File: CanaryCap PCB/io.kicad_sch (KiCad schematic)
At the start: 15 parts, among them J1 USB_C_Receptacle_USB2.0_16P, J2 Conn_01x06_Pin, J3 Conn_01x04_Pin, U5 ADXL343

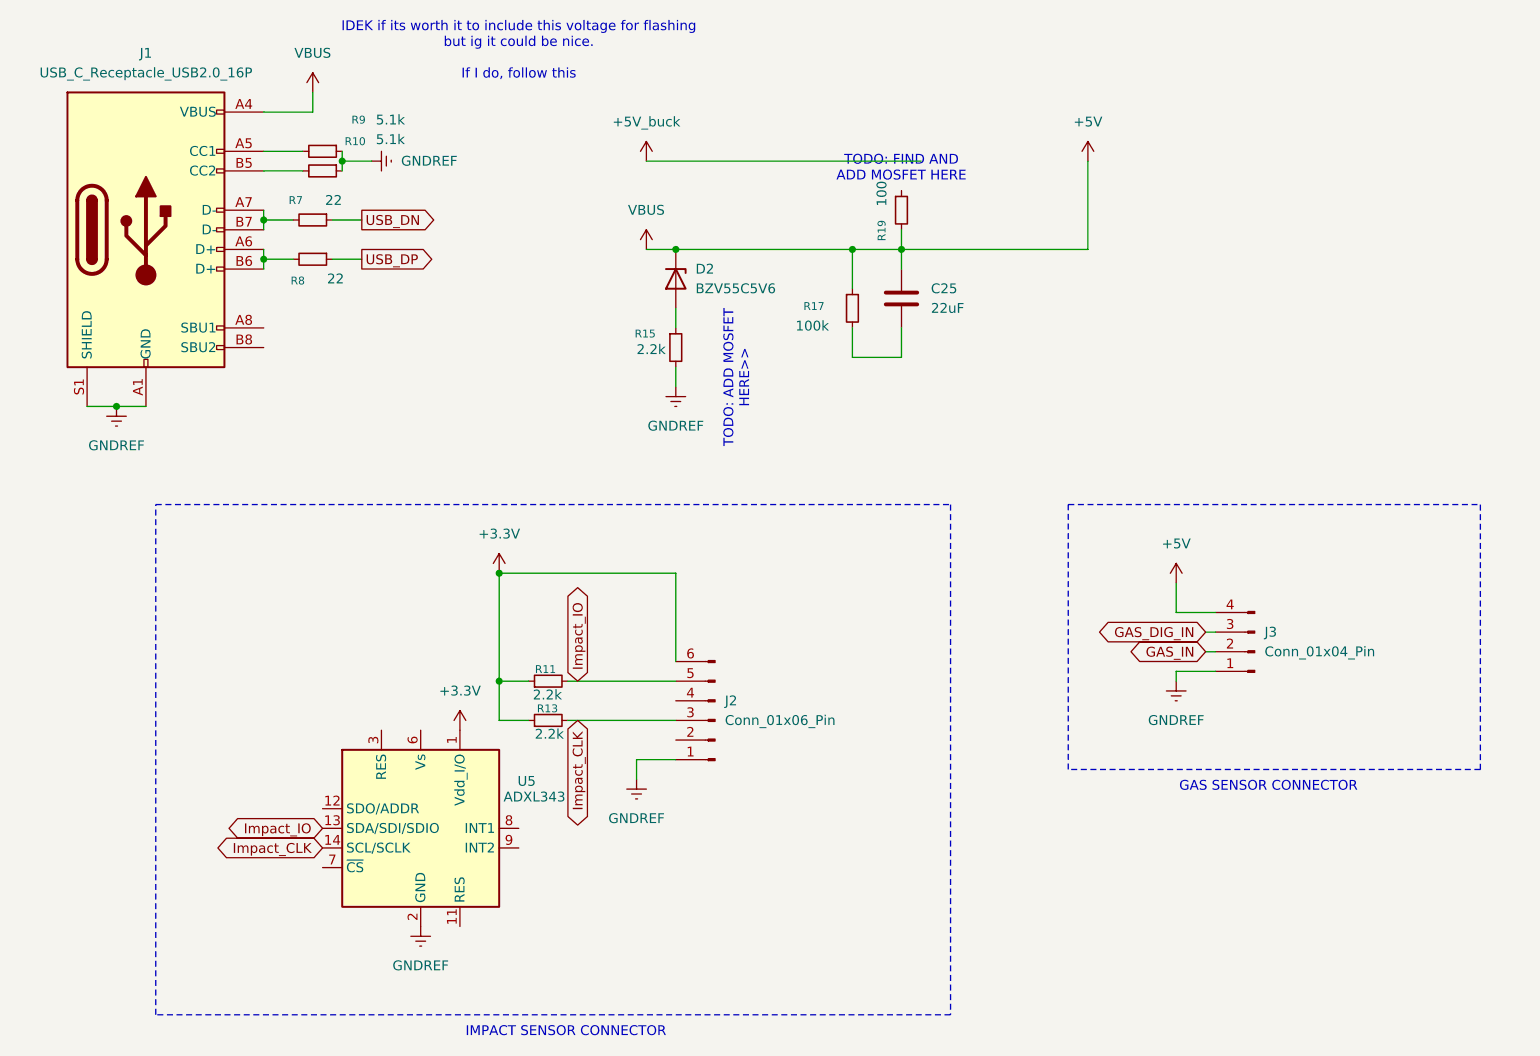
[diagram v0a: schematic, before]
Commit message: FIXED IT MF
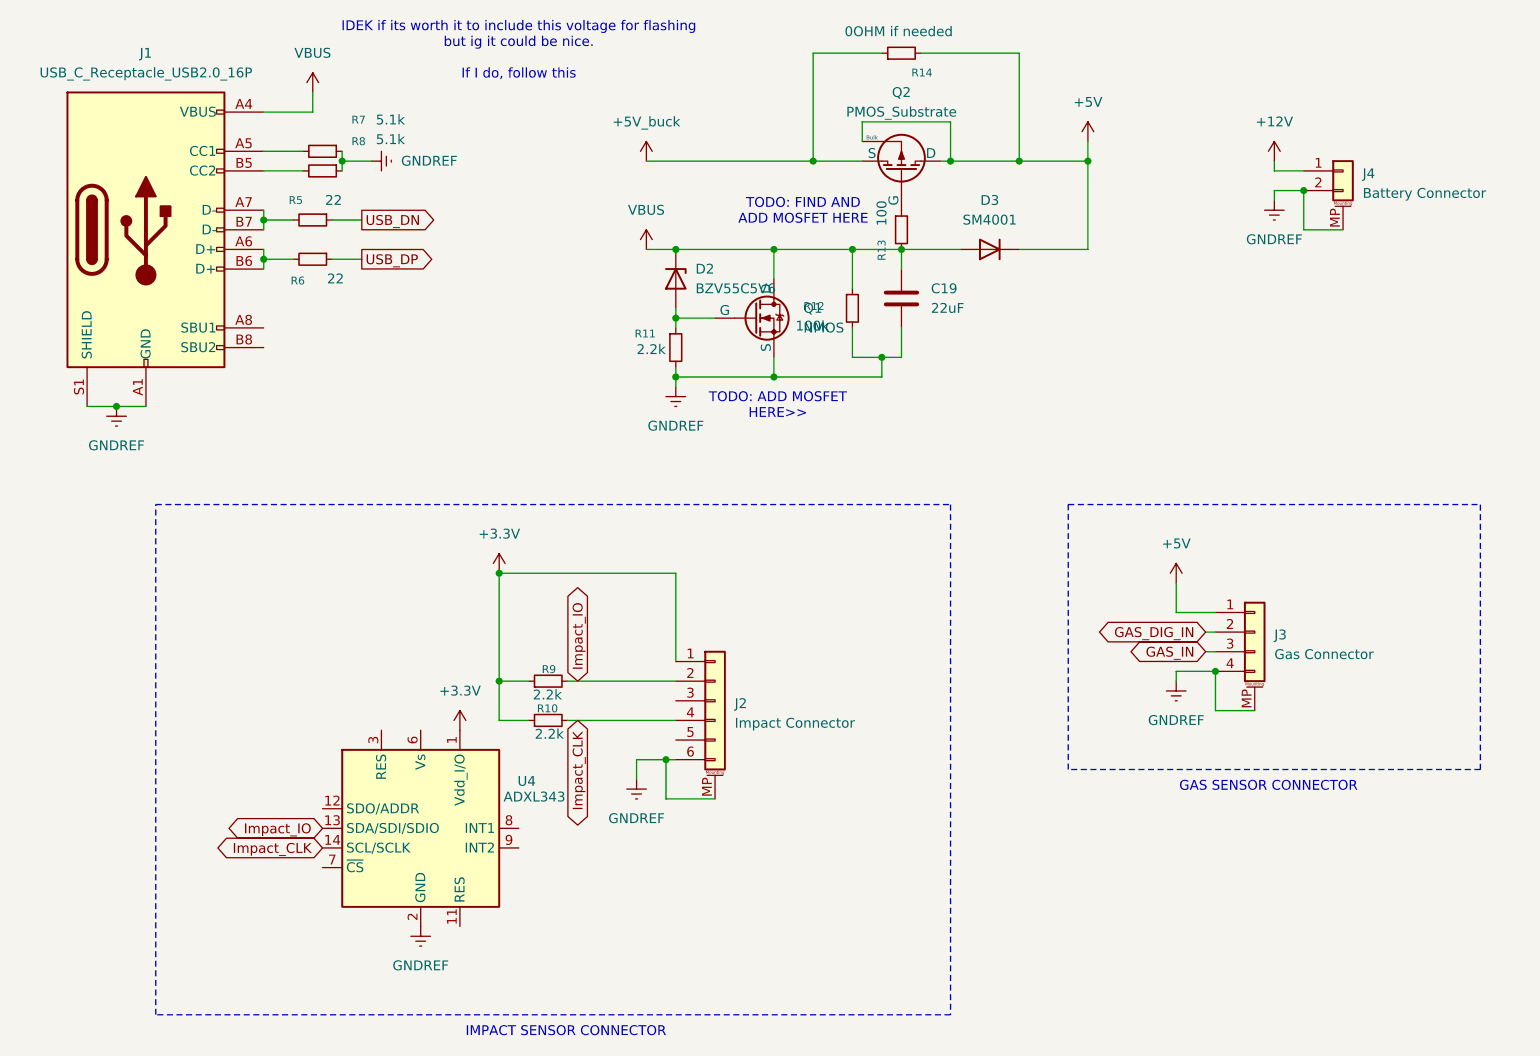
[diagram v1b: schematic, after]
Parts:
- removed J2: Conn_01x06_Pin, Connector_IDC:IDC-Header_2x03_P2.54mm_Vertical, symbol Connector:Conn_01x06_Pin
- removed J3: Conn_01x04_Pin, Connector_PinHeader_1.00mm:PinHeader_2x02_P1.00mm_Vertical, symbol Connector:Conn_01x04_Pin
- added D3: SM4001, Diode_SMD:D_MELF, symbol Diode:SM4001
- added J2: Impact Connector, Connector_Molex:Molex_CLIK-Mate_502443-0670_1x06-1MP_P2.00mm_Vertical, symbol Connector_Generic_MountingPin:Conn_01x06_MountingPin
- added J3: Gas Connector, Connector_Molex:Molex_CLIK-Mate_502443-0470_1x04-1MP_P2.00mm_Vertical, symbol Connector_Generic_MountingPin:Conn_01x04_MountingPin
- added J4: Battery Connector, Connector_Molex:Molex_CLIK-Mate_502443-0270_1x02-1MP_P2.00mm_Vertical, symbol Connector_Generic_MountingPin:Conn_01x02_MountingPin
- added Q1: NMOS, Package_TO_SOT_SMD:SOT-23, symbol Simulation_SPICE:NMOS
- added Q2: PMOS_Substrate, Package_TO_SOT_SMD:SOT-223, symbol Simulation_SPICE:PMOS_Substrate
- added R14: 0OHM if needed, Resistor_SMD:R_0603_1608Metric_Pad0.98x0.95mm_HandSolder, symbol Device:R_Small
- renumbered C25 to C19, R13 to R10, R15 to R11, R17 to R12, R19 to R13, R7 to R5, R8 to R6, R9 to R7, R10 to R8, R11 to R9, U5 to U4
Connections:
- net +3.3V: now also J2.1 (Pin_1)
- net +5V: now also D3.1 (K), J3.1 (Pin_1), Q2.2 (D), Q2.4 (Bulk), R14.2; no longer C19.1, D2.1 (K), J1.A4 (VBUS), J1.A9 (VBUS), J1.B4 (VBUS), J1.B9 (VBUS), R12.1, R13.2
- net +5V_buck: now also Q2.3 (S), R14.1
- net GAS_DIG_IN: now also J3.2 (Pin_2)
- net GAS_IN: now also J3.3 (Pin_3)
- net GNDREF: now also C19.2, R12.2, J2.6 (Pin_6), J2.MP (MountPin), J3.4 (Pin_4), J3.MP (MountPin), J4.2 (Pin_2), J4.MP (MountPin), Q1.2 (S)
- net Impact_CLK: now also J2.4 (Pin_4)
- net Impact_IO: now also J2.2 (Pin_2)
- net at D2.2 (A), R11.1: now also Q1.1 (G)
- net at R13.1: now also Q2.1 (G)
- new net +12V: J4.1 (Pin_1)
- new net VBUS: C19.1, D2.1 (K), D3.2 (A), J1.A4 (VBUS), J1.A9 (VBUS), J1.B4 (VBUS), J1.B9 (VBUS), Q1.3 (D), R12.1, R13.2
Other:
- moved on the sheet: R13

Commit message: Added todo
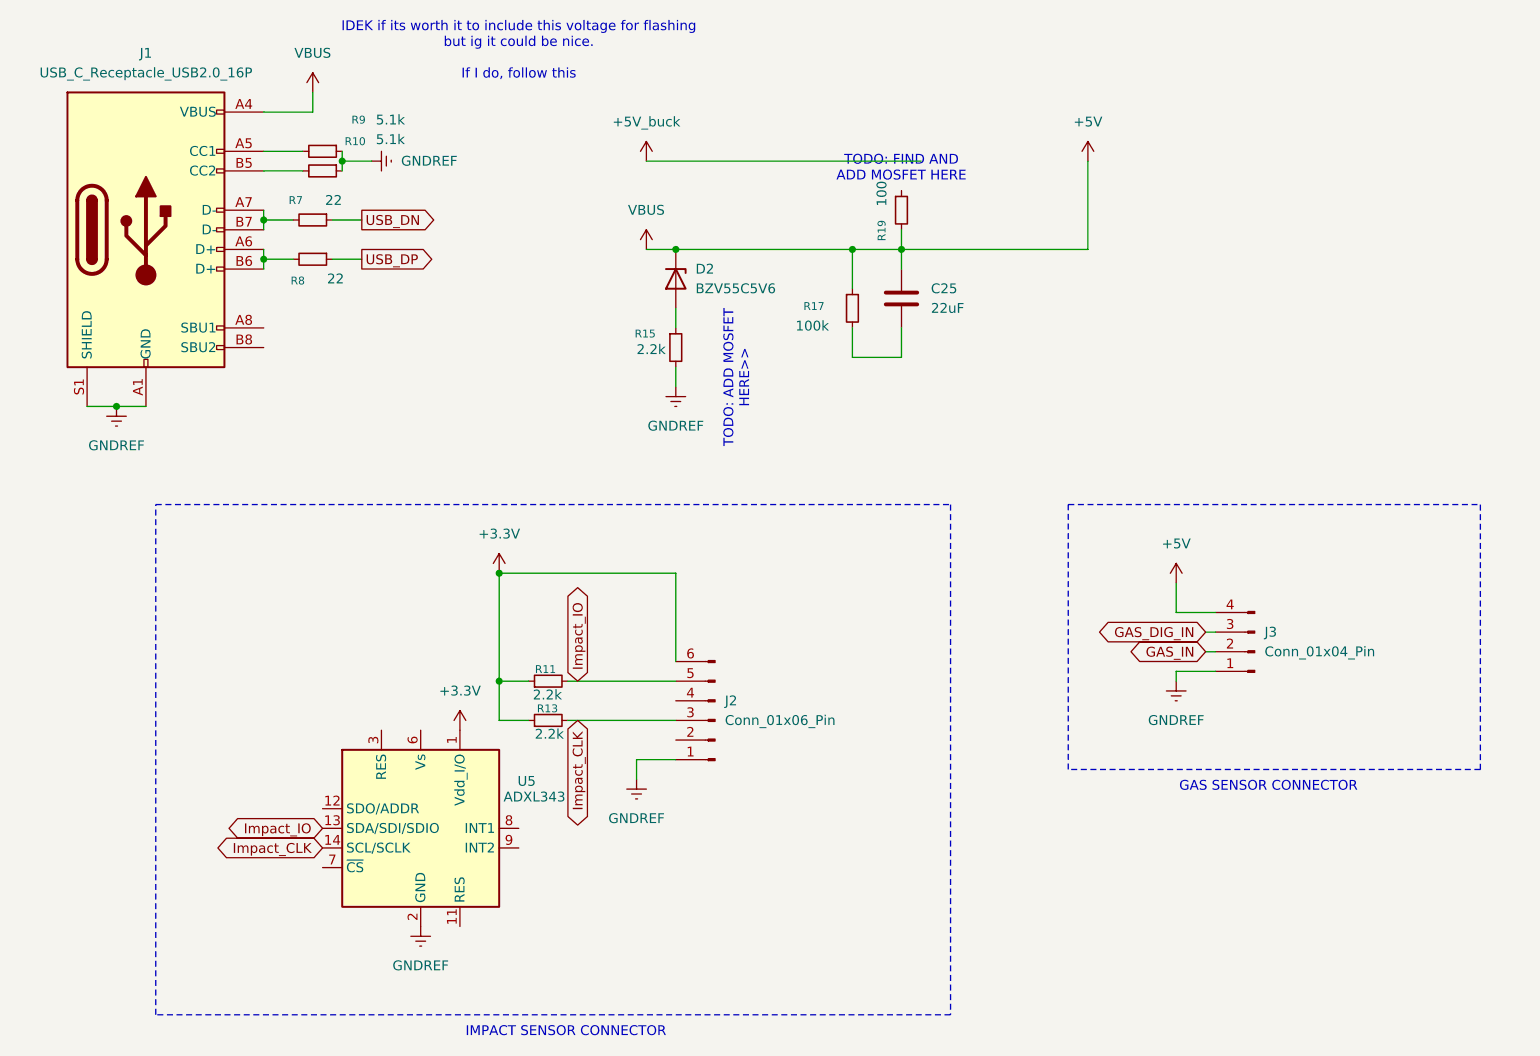
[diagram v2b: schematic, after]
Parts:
- removed D3: SM4001, Diode_SMD:D_MELF, symbol Diode:SM4001
- removed J2: Impact Connector, Connector_Molex:Molex_CLIK-Mate_502443-0670_1x06-1MP_P2.00mm_Vertical, symbol Connector_Generic_MountingPin:Conn_01x06_MountingPin
- removed J3: Gas Connector, Connector_Molex:Molex_CLIK-Mate_502443-0470_1x04-1MP_P2.00mm_Vertical, symbol Connector_Generic_MountingPin:Conn_01x04_MountingPin
- removed J4: Battery Connector, Connector_Molex:Molex_CLIK-Mate_502443-0270_1x02-1MP_P2.00mm_Vertical, symbol Connector_Generic_MountingPin:Conn_01x02_MountingPin
- removed Q1: NMOS, Package_TO_SOT_SMD:SOT-23, symbol Simulation_SPICE:NMOS
- removed Q2: PMOS_Substrate, Package_TO_SOT_SMD:SOT-223, symbol Simulation_SPICE:PMOS_Substrate
- removed R14: 0OHM if needed, Resistor_SMD:R_0603_1608Metric_Pad0.98x0.95mm_HandSolder, symbol Device:R_Small
- added J2: Conn_01x06_Pin, Connector_IDC:IDC-Header_2x03_P2.54mm_Vertical, symbol Connector:Conn_01x06_Pin
- added J3: Conn_01x04_Pin, Connector_PinHeader_1.00mm:PinHeader_2x02_P1.00mm_Vertical, symbol Connector:Conn_01x04_Pin
- renumbered C19 to C25, R8 to R10, R9 to R11, R10 to R13, R11 to R15, R12 to R17, R13 to R19, R5 to R7, R6 to R8, R7 to R9, U4 to U5
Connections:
- net VBUS is gone; now on net +5V: C25.1, D2.1 (K), J1.A4 (VBUS), J1.A9 (VBUS), J1.B4 (VBUS), J1.B9 (VBUS), R17.1, R19.2
- net +3.3V: now also J2.6 (Pin_6)
- net +5V: now also J3.4 (Pin_4)
- net GAS_DIG_IN: now also J3.3 (Pin_3)
- net GAS_IN: now also J3.2 (Pin_2)
- net GNDREF: now also J2.1 (Pin_1), J3.1 (Pin_1); no longer C25.2, R17.2
- net Impact_CLK: now also J2.3 (Pin_3)
- net Impact_IO: now also J2.5 (Pin_5)
- new net: C25.2, R17.2
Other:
- moved on the sheet: R19
